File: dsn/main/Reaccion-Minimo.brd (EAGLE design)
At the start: 102.9 x 40.6 mm, 43 parts, among them U1 ATMEGA328P_TQFP, U2 MIC5219 5V, Y1 16MHz

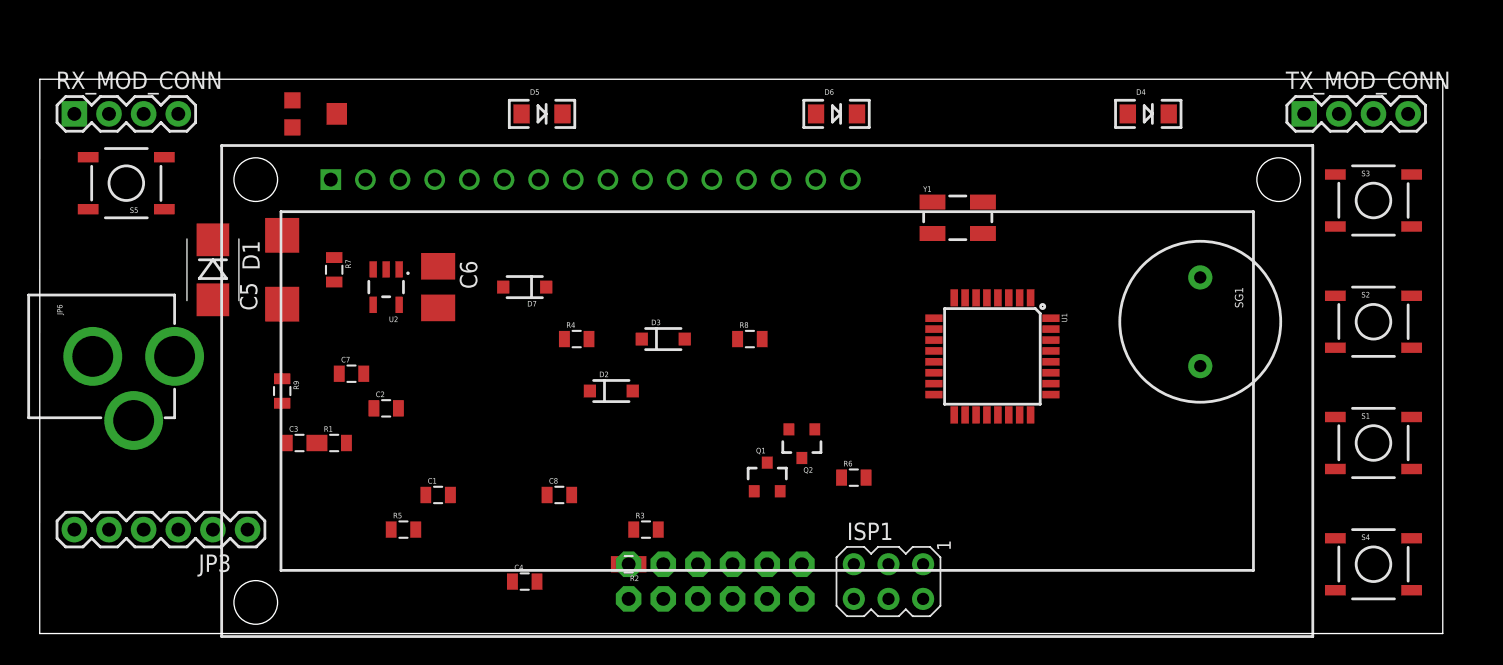
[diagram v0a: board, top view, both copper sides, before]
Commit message: Added Reaccion-Minimo PASTO
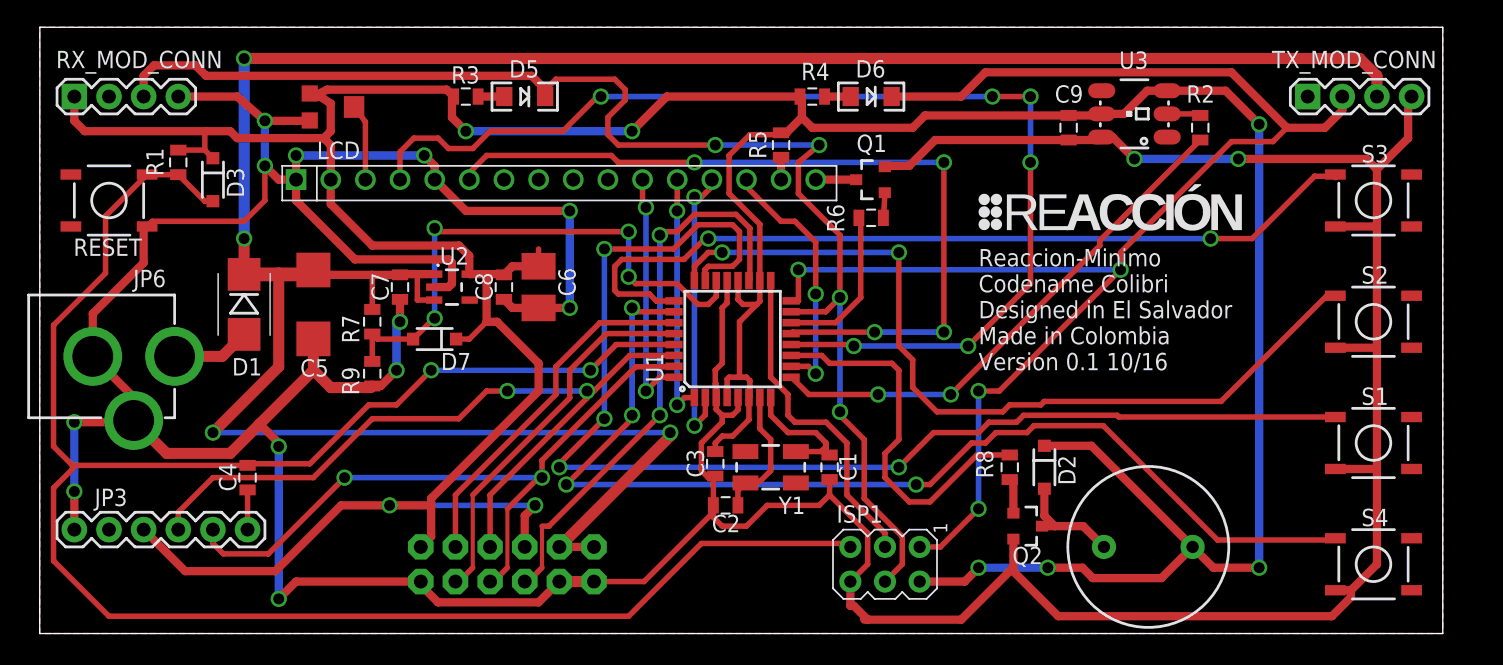
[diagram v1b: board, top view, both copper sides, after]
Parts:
- removed D4: GREEN, SparkFun-LED:LED-1206
- removed S5: SWITCH-MOMENTARY-2SMD, SparkFun-Electromechanical:TACTILE-SWITCH-SMD
- removed U$1: LCD-HD447803-HOLES16X2-3-HOLES, HD44780LCD:LCD-16X2-3HOLES
- added C9: 1uF, SparkFun-Capacitors:0805
- added LCD: LCD-HD447803-HOLES16X2-3-HOLES, HD44780LCD:LCD-16X2-3HOLES
- added RESET: SWITCH-MOMENTARY-2SMD, SparkFun-Electromechanical:TACTILE-SWITCH-SMD
- added U3: WS2811, SparkFun-LED:LED-TRICOLOR-5050-IC
- C1, C2: value (none) -> 18pF
- C3, C7: value (none) -> 1uF
- C4: value (none) -> 0.1uF
- C6: value (none) -> 100uF
- C8: value (none) -> 4.7uF
- R1, R6, R8: value (none) -> 4.7K
- R2: value (none) -> 150
- R3, R4: value (none) -> 330
- R5: value (none) -> 0
- U2: value MIC5219 5V -> lp2992aim5-5.0
- moved R2 52.7 mm to (85.1, 37.1), turned to 270 degrees
- moved R5 39.5 mm to (54.4, 35.8), turned to 90 degrees
- moved D3 35.0 mm to (12.7, 33.3), turned to 270 degrees
- moved R3 34.4 mm to (31.2, 39.4), turned to 180 degrees
- moved D2 32.2 mm to (73.7, 12.2), turned to 270 degrees
- moved C3 30.5 mm to (49.5, 12.4), turned to 90 degrees
- moved C1 28.8 mm to (57.9, 12.2), turned to 90 degrees
- moved C2 25.9 mm to (50.3, 9.40)
- moved R4 24.8 mm to (56.6, 39.4), turned to 180 degrees
- moved R1 23.5 mm to (10.2, 34.5), turned to 90 degrees
- moved Q1 23.1 mm to (61.0, 33.3), turned to 90 degrees
- moved Y1 22.9 mm to (53.6, 12.2), turned to 180 degrees
- moved C4 21.7 mm to (15.2, 11.4), turned to 90 degrees
- moved R8 21.2 mm to (71.1, 12.2), turned to 270 degrees
- moved R6 19.1 mm to (61.0, 30.5), turned to 180 degrees
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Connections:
- net 5V: now also C9.2, LCD.2, U3.3, U3.5; no longer R2.2, U$1.2
- net D2: now also LCD.11; no longer U$1.11
- net D3: now also LCD.12; no longer U$1.12
- net D4: now also LCD.13; no longer U$1.13
- net D6: now also LCD.14; no longer U$1.14
- net D8: now also LCD.4; no longer U$1.4
- net D9: now also LCD.6; no longer U$1.6
- net GND: now also C9.1, LCD.1, LCD.5, RESET.1, U3.6; no longer S5.1, U$1.1, U$1.5
- net HEARTBEAT: now also R2.2; no longer D4.C
- net N$3: now also U3.2; no longer D4.A
- net N$6: now also LCD.15; no longer U$1.15
- net N$7: now also LCD.3; no longer U$1.3
- net N$8: now also LCD.16; no longer U$1.16
- net RESET: now also RESET.3; no longer S5.3
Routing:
- net GND: track 0.00 -> 364.9 mm, vias 0 -> 14
- net 5V: track 0.00 -> 308.0 mm, vias 0 -> 8
- net VIN_RECT: track 0.00 -> 182.3 mm, vias 0 -> 4
- net RESET: track 0.00 -> 148.3 mm, vias 0 -> 2
- net RF_TX: track 0.00 -> 108.9 mm, vias 0 -> 4
- net RF_RX: track 0.00 -> 99.1 mm, vias 0 -> 4
- net BTN_BUS0: track 0.00 -> 92.4 mm, vias 0 -> 4
- net D8: track 0.00 -> 83.8 mm, vias 0 -> 6
- net BTN_BUS3: track 0.00 -> 79.9 mm, vias 0 -> 4
- net BTN_BUS2: track 0.00 -> 62.1 mm, vias 0 -> 2
- net BTN_BUS1: track 0.00 -> 62.0 mm, vias 0 -> 2
- net D9: track 0.00 -> 59.7 mm, vias 0 -> 4
- net RX: track 0.00 -> 56.8 mm, vias 0 -> 2
- net TX: track 0.00 -> 51.1 mm, vias 0 -> 2
- net ADC6: track 0.00 -> 41.5 mm, vias 0 -> 2
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- added copper zone on layer 1, net GND
- added copper zone on layer 16, net GND
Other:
- board size 102.9 x 40.6 mm -> 102.9 x 44.5 mm
- board text added: "Galeras volcano. Artwork generated from Jorge Luis Recalde Mesías photo CC BY-SA 3.0"
- board text added: "Reaccion-Minimo Codename Colibri Designed in El Salvador Made in Colombia Version 0.1 10/16"
